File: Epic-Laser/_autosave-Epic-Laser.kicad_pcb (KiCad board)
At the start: 2 copper layers, 10 parts, among them J1 ICSP-Header, U1 PIC24FJ64GA002-I_SP, X1 USB-B1HSB6

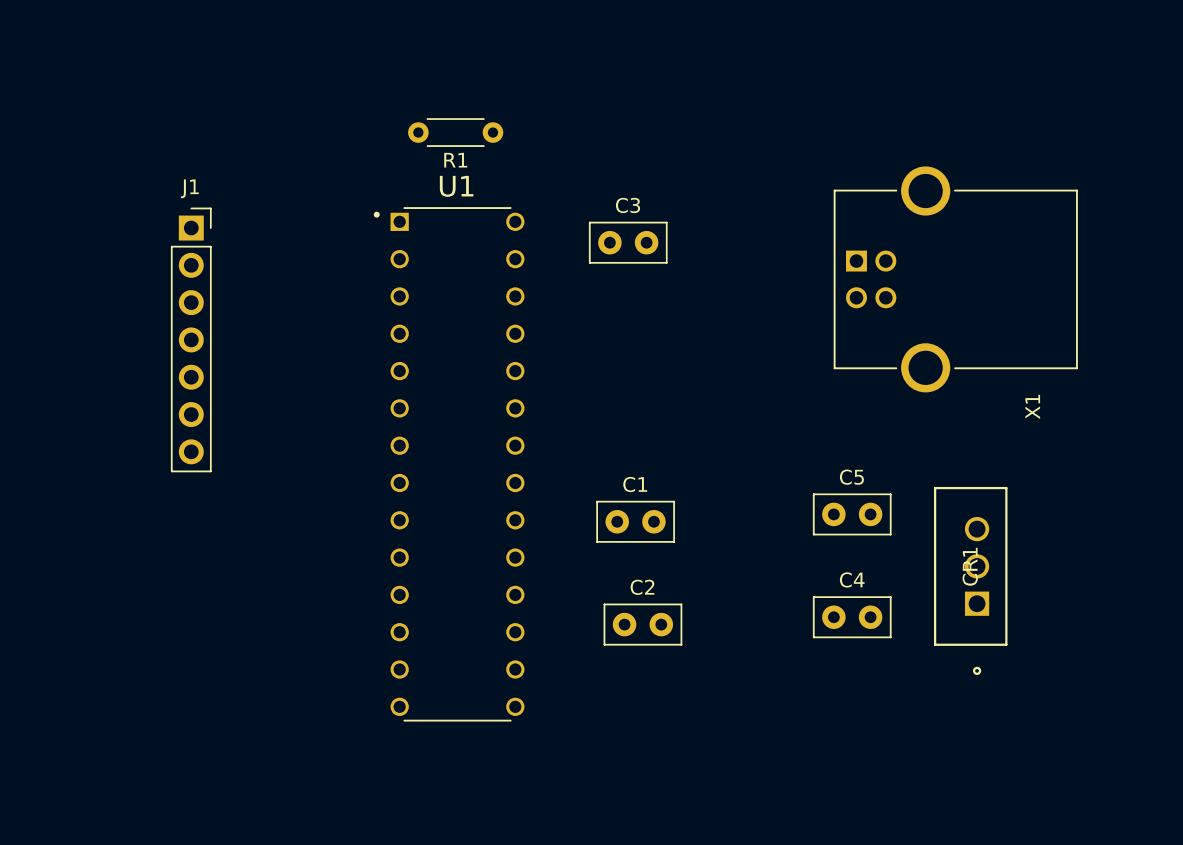
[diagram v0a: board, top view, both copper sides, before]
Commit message: Draft-Schematics
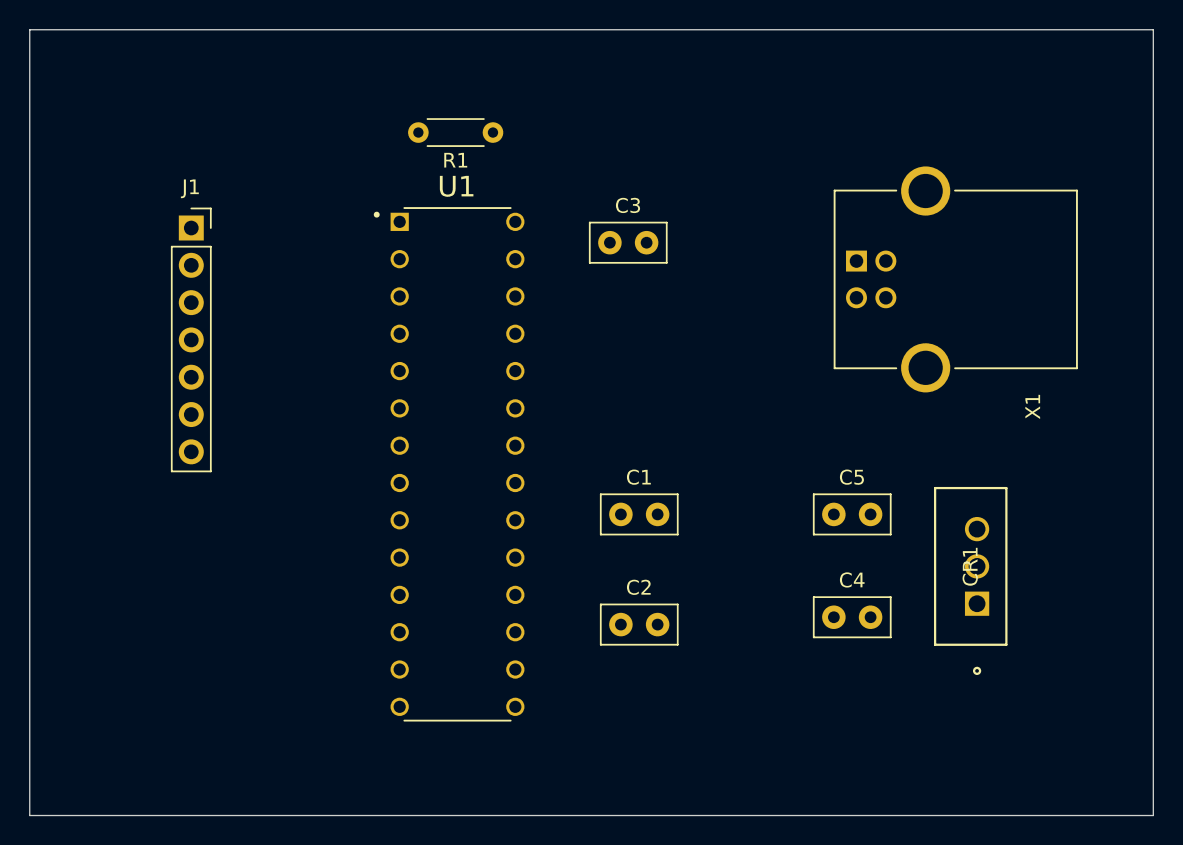
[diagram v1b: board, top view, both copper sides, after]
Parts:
- moved C1 0.56 mm to (145.2, 88.0)
- moved C2 0.25 mm to (145.2, 95.5)
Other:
- board outline added: 76.5 x 53.5 mm
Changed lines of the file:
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@@
 	(footprint "Capacitor_THT:C_Disc_D5.0mm_W2.5mm_P2.50mm"
 		(layer "F.Cu")
-		(at 145.5 95.5)
+		(at 145.25 95.5)
 		(descr "C, Disc series, Radial, pin pitch=2.50mm, diameter*width=5*2.5mm^2, Capacitor, http://cdn-reichelt.de/documents/datenblatt/B300/DS_KERKO_TC.pdf")
 		(tags "C Disc series Radial pin pitch 2.50mm diameter 5mm width 2.5mm Capacitor")
@@
 	(footprint "Capacitor_THT:C_Disc_D5.0mm_W2.5mm_P2.50mm"
 		(layer "F.Cu")
-		(at 145 88.5)
+		(at 145.25 88)
 		(descr "C, Disc series, Radial, pin pitch=2.50mm, diameter*width=5*2.5mm^2, Capacitor, http://cdn-reichelt.de/documents/datenblatt/B300/DS_KERKO_TC.pdf")
 		(tags "C Disc series Radial pin pitch 2.50mm diameter 5mm width 2.5mm Capacitor")
@@
 		)
 		(embedded_fonts no)
+		(model "/Users/samuel/Documents/KiCad-Tools/3D-models/PIC24FJ64GA002-I_SP.step"
+			(offset
+				(xyz 0 0 0)
+			)
+			(scale
+				(xyz 1 1 1)
+			)
+			(rotate
+				(xyz -90 -0 -0)
+			)
+		)
 	)
 	(footprint "Resistor_THT:R_Axial_DIN0204_L3.6mm_D1.6mm_P5.08mm_Horizontal"
@@
 		)
 	)
+	(gr_rect
+		(start 105 55)
+		(end 181.5 108.5)
+		(stroke
+			(width 0.05)
+			(type default)
+		)
+		(fill no)
+		(layer "Edge.Cuts")
+	)
 	(embedded_fonts no)
